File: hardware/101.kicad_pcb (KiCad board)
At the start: 2 copper layers, 0 parts

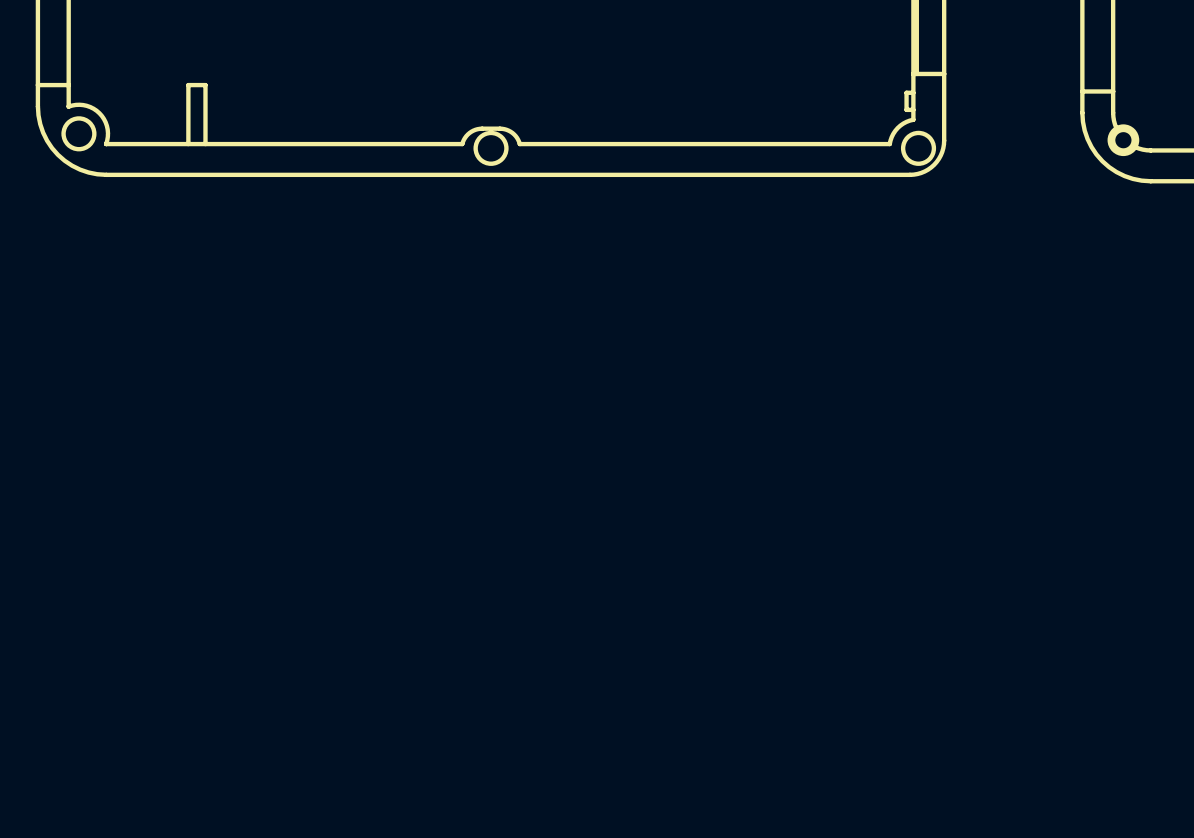
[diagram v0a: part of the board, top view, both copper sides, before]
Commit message: add: 随便画了画pcb
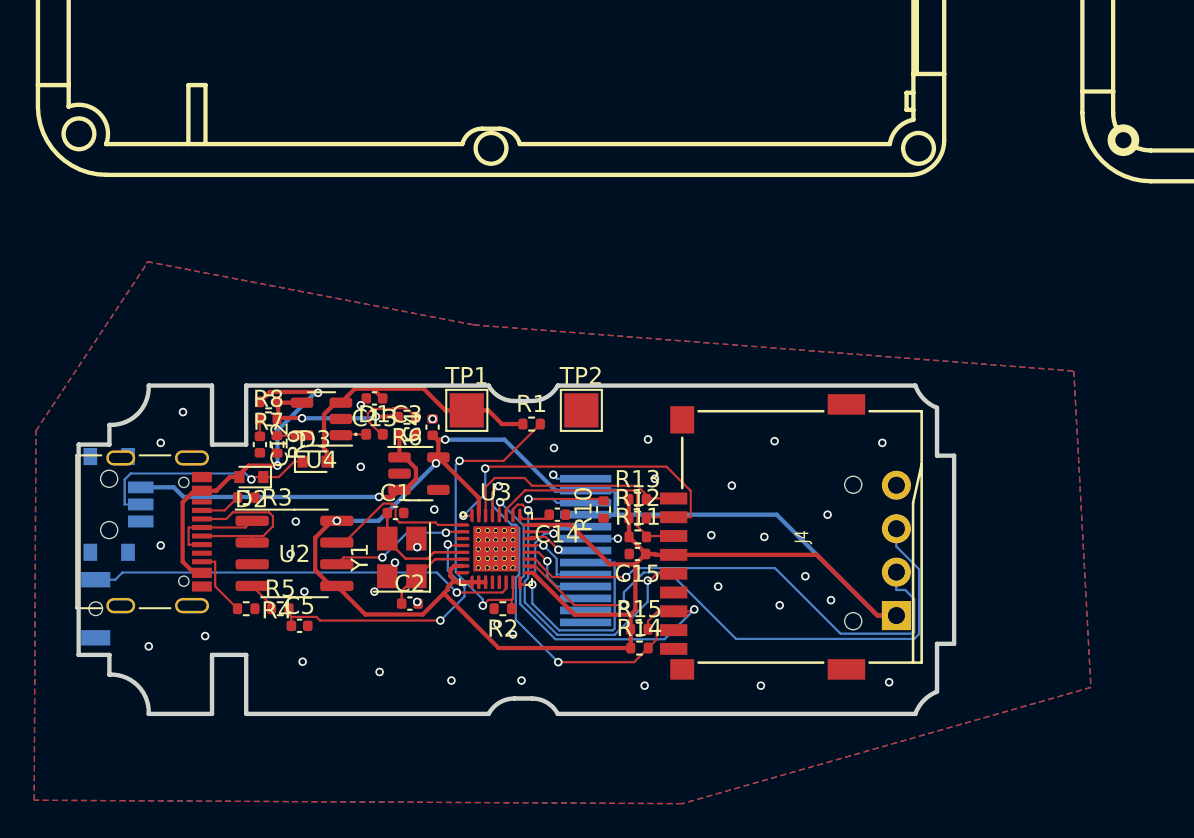
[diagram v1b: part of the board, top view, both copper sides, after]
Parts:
- added C1: 15p, Capacitor_SMD:C_0402_1005Metric, F.Cu at (36.7, 58.3)
- added C12: 1uF, Capacitor_SMD:C_0402_1005Metric, F.Cu at (28.8, 54.3)
- added C13: 1uF, Capacitor_SMD:C_0402_1005Metric, F.Cu at (35.5, 51.6)
- added C14: 4.7uF, Capacitor_SMD:C_0402_1005Metric, F.Cu at (46.2, 58.4)
- added C15: 100nf, Capacitor_SMD:C_0402_1005Metric, F.Cu at (50.9, 60.7)
- added C2: 15p, Capacitor_SMD:C_0402_1005Metric, F.Cu at (37.6, 63.6)
- added C3: 1uF, Capacitor_SMD:C_0402_1005Metric, F.Cu at (37.4, 53.7)
- added C4: 1uF, Capacitor_SMD:C_0402_1005Metric, F.Cu at (38.9, 53.3)
- added C5: 100nf, Capacitor_SMD:C_0402_1005Metric, F.Cu at (31.1, 64.9)
- added D1: LED, LED_SMD:LED_0402_1005Metric, F.Cu at (35.5, 53.7)
- added D2: MSK4005, Diode_SMD:D_SOD-523, F.Cu at (28.3, 56.2)
- added D3: MSK4005, Diode_SMD:D_SOD-523, F.Cu at (32.0, 55.3)
- added J1: USB_C_Receptacle_USB2.0, Connector_USB:USB_C_Receptacle_Palconn_UTC16-G, F.Cu at (22.9, 59.4)
- added J2: Conn_01x04_Male, Connector_PinHeader_2.54mm:PinHeader_1x04_P2.54mm_Horizontal, B.Cu at (66.0, 64.3)
- added J3: ST7735S-0.96TFT-13P, chenxuuu_Module:ST7735S-0.96TFT-13P, B.Cu at (46.6, 60.5)
- added J4: Micro_SD_Card, chenxuuu_Module:microSD_TF, F.Cu at (60.5, 59.7)
- added R1: 100K, Resistor_SMD:R_0402_1005Metric, F.Cu at (44.7, 53.1)
- added R10: 10R, Resistor_SMD:R_0402_1005Metric, F.Cu at (48.9, 58.1)
- added R11: 100K, Resistor_SMD:R_0402_1005Metric, F.Cu at (50.9, 59.7)
- added R12: 100K, Resistor_SMD:R_0402_1005Metric, F.Cu at (50.9, 58.6)
- added R13: 100K, Resistor_SMD:R_0402_1005Metric, F.Cu at (50.9, 57.5)
- added R14: 100K, Resistor_SMD:R_0402_1005Metric, F.Cu at (51.0, 66.2)
- added R15: 100K, Resistor_SMD:R_0402_1005Metric, F.Cu at (51.0, 65.1)
- added R2: 100K, Resistor_SMD:R_0402_1005Metric, F.Cu at (43.0, 63.9)
- added R3: 5.1K, Resistor_SMD:R_0402_1005Metric, F.Cu at (28.0, 57.4)
- added R4: 5.1K, Resistor_SMD:R_0402_1005Metric, F.Cu at (28.0, 63.9)
- added R5: 5.1K, Resistor_SMD:R_0402_1005Metric, F.Cu at (30.0, 63.9)
- added R6: 1K, Resistor_SMD:R_0402_1005Metric, F.Cu at (37.4, 52.7)
- added R7: 0.5R, Resistor_SMD:R_0402_1005Metric, F.Cu at (29.3, 51.8)
- added R8: 1R, Resistor_SMD:R_0402_1005Metric, F.Cu at (29.3, 52.8)
- added R9: 2K, Resistor_SMD:R_0402_1005Metric, F.Cu at (29.8, 54.3)
- added SW1: Side_SWITCH_SW_3*6*3.5mm, Button_Switch_SMD:SW_SPST_B3U-3000P-B, B.Cu at (19.2, 63.9)
- added SW2: SW_Push_SPDT, chenxuuu_Module:MSK-0002, B.Cu at (20.0, 57.8)
- added TP1: TestPoint, TestPoint:TestPoint_Pad_2.0x2.0mm, F.Cu at (40.9, 52.3)
- added TP2: TestPoint, TestPoint:TestPoint_Pad_2.0x2.0mm, F.Cu at (47.6, 52.3)
- added U1: 4A2D, Package_TO_SOT_SMD:SOT-23-5, F.Cu at (38.1, 56.0)
- added U2: CH330N, Package_SO:SOIC-8_3.9x4.9mm_P1.27mm, F.Cu at (30.8, 60.7)
- added U3: Air101, Air_LuatOS_Module:Air101, F.Cu at (42.6, 60.4)
- added U4: HX4064A, Package_TO_SOT_SMD:SOT-23-5, F.Cu at (32.4, 52.8)
- added Y1: 40M, Crystal:Crystal_SMD_3225-4Pin_3.2x2.5mm, F.Cu at (37.1, 60.9)
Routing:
- net +3V3: track 0.00 -> 116.4 mm, vias 0 -> 3
- net /UART3_RX: track 0.00 -> 33.4 mm, vias 0 -> 1
- net /UART3_TX: track 0.00 -> 29.1 mm, vias 0 -> 1
- net /KEY: track 0.00 -> 25.0 mm, vias 0 -> 1
- net /TF_DAT0: track 0.00 -> 22.6 mm, vias 0 -> 2
- net /TF_DAT1: track 0.00 -> 22.1 mm, vias 0 -> 2
- net /TF_DAT3: track 0.00 -> 20.6 mm, vias 0 -> 2
- net +5V: track 0.00 -> 20.4 mm, vias 0 -> 2
- net Net-(C3-Pad1): track 0.00 -> 20.0 mm, vias 0 -> 1
- net /TF_CLK: track 0.00 -> 18.7 mm, vias 0 -> 2
- net Net-(R1-Pad2): track 0.00 -> 18.2 mm, vias 0 -> 2
- net +4V: track 0.00 -> 16.7 mm
- net /RESET: track 0.00 -> 16.2 mm, vias 0 -> 2
- net /TF_DAT2: track 0.00 -> 13.6 mm
- net /LDO_IN: track 0.00 -> 13.5 mm, vias 0 -> 1
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- added copper zone on B.Cu, net GND
- added copper zone on F.Cu, net GND
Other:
- board outline added: 51.2 x 19.2 mm
